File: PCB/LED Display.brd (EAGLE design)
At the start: 62 x 42.5 mm, 38 parts, among them IC1 LM2596S, IC2 LTC485S, IC3 MEGA32-A, X1 RJ45-6L21-B

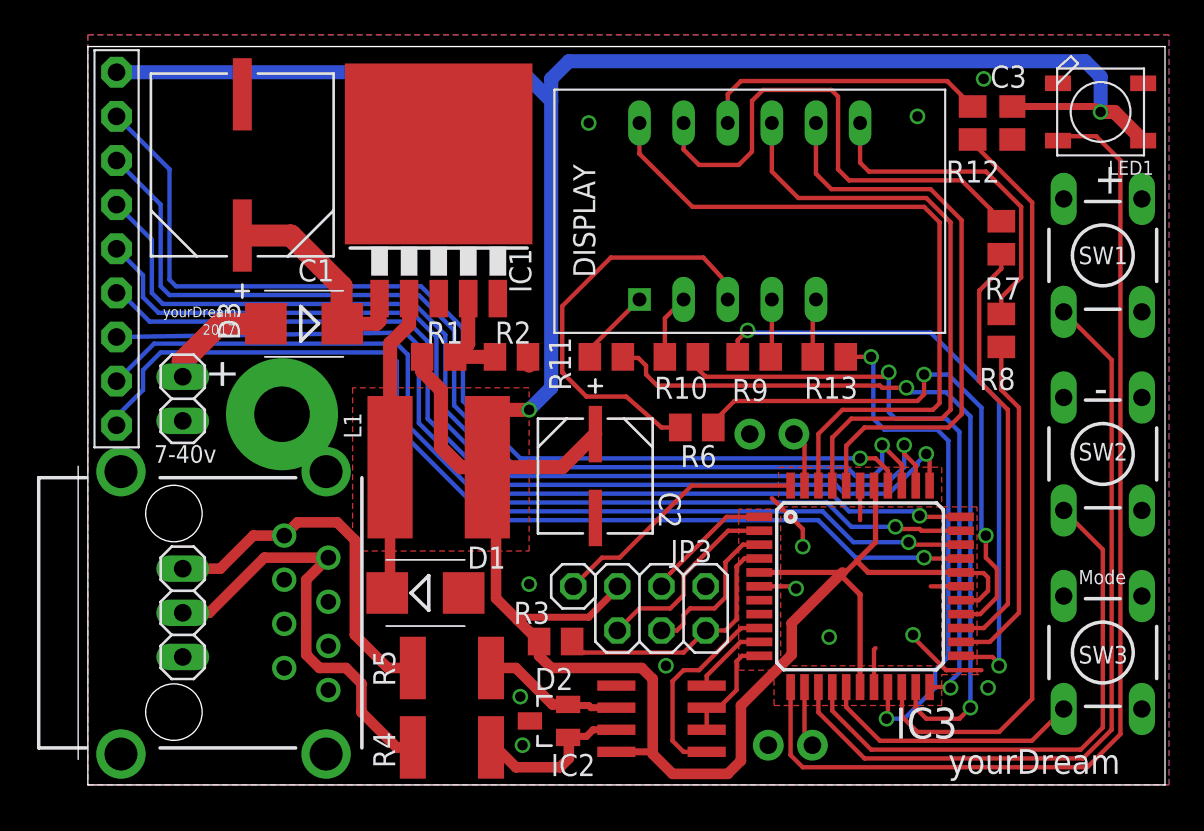
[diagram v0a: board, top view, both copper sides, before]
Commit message: Numerous fixes.
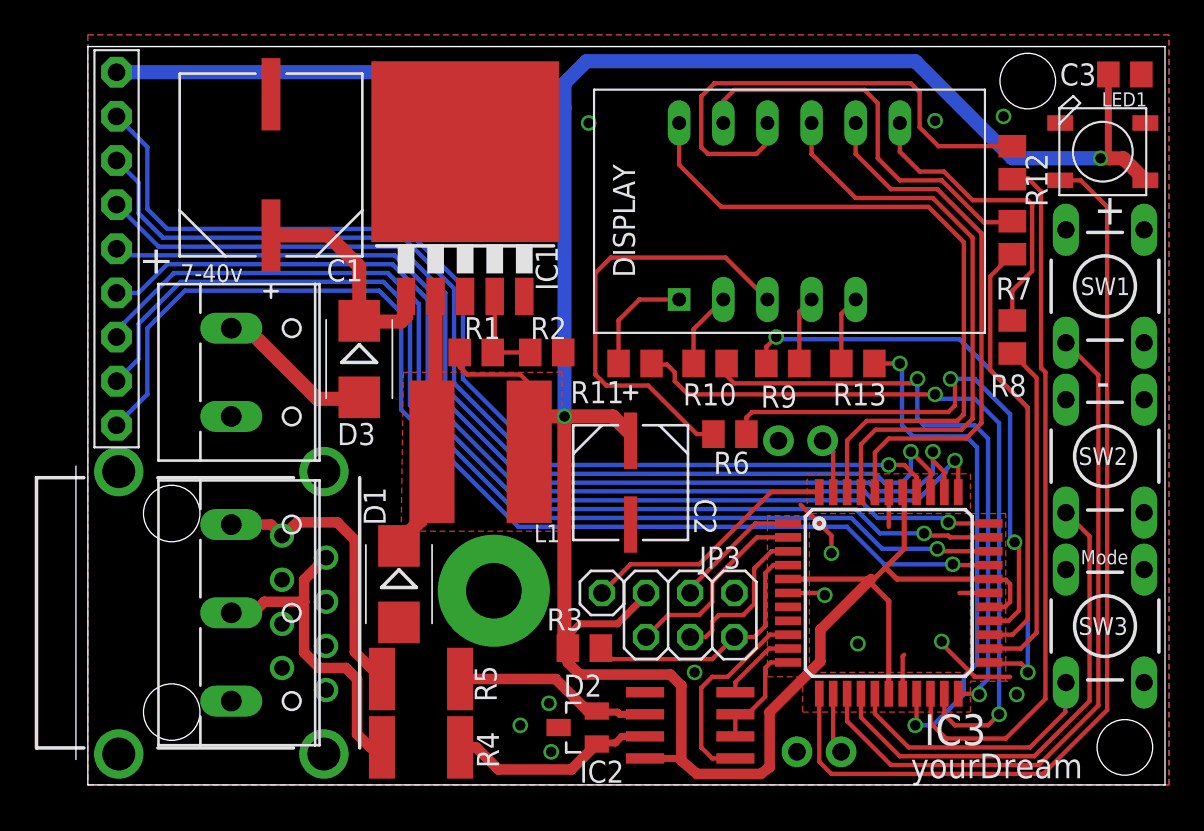
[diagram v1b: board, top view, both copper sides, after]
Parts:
- removed DMX: DMX, pinhead:1X03
- removed POWER: 7-40V, pinhead:1X02
- added X2: (no value), con-wago-508:W237-132
- added X3: (no value), con-wago-508:W237-133
- moved - 11.6 mm to (58.5, 18.9)
- moved + 9.65 mm to (58.5, 28.7)
- moved C3 7.05 mm to (59.7, 40.9), turned to 0 degrees
- moved D3 3.77 mm to (15.6, 24.5), turned to 270 degrees
- moved R12 3.23 mm to (53.2, 35.8)
- moved U$1 2.57 mm to (22.6, 19.2)
- moved LED1 2.29 mm to (58.4, 36.4)
- moved DISPLAY 2.29 mm to (40.4, 33.0)
- moved R1 2.17 mm to (22.4, 24.9)
- moved C2 2.07 mm to (31.2, 17.4)
- moved R2 2.05 mm to (26.4, 24.9)
- moved R6 1.94 mm to (37.0, 20.2)
- moved R5 1.89 mm to (19.2, 6.10)
- moved R4 1.78 mm to (19.2, 2.16)
- moved JP2 1.69 mm to (40.8, 1.91)
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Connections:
- net GND: now also X2.2, X3.3; no longer DMX.3, POWER.1
- net N$10: now also X3.1; no longer DMX.1
- net N$14: now also +.1; no longer -.1
- net N$26: now also -.1; no longer +.1
- net N$41: now also X2.1; no longer POWER.2
- net N$9: now also X3.2; no longer DMX.2
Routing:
- net N$16: track 16.7 -> 29.2 mm
- net PA7: track 58.4 -> 65.5 mm
- net PA6: track 56.8 -> 63.6 mm
- net DI: track 61.2 -> 54.6 mm
- net N$9: track 25.1 -> 19.0 mm
- net N$21: track 29.3 -> 23.2 mm
- net PA5: track 56.1 -> 61.8 mm
- net N$14: track 45.3 -> 40.2 mm
- net N$10: track 21.0 -> 16.7 mm
- net PA4: track 56.5 -> 60.4 mm
- net N$26: track 31.8 -> 28.2 mm
- net N$5: track 8.28 -> 11.6 mm
- net +5V: track 189.5 -> 186.4 mm
- net N$31: track 44.0 -> 40.9 mm
- net N$2: track 9.35 -> 12.0 mm
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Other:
- board text removed: "2017"
